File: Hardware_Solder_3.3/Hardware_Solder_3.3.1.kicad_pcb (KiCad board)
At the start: 2 copper layers, 86.5 x 47.4 mm, 95 parts, among them J1 Connector, J2 POWER, J3 SENSOR, J4 BATTERY, J5 Control Panel, J6 SWD DEBUG, J7 HEAT_WIRE, Q1 S8050, Q2 S8050, Q3 S8550, Q4 IRFS4227, Q6 S8050, SW1 RESET, U1 LM358, U2 W25Q32JVSS, U3 LM2596S-ADJ, U4 ACS712-05A, U5 AMS1117-3.3, U6 STM32F103C8Tx, Y1 32.768KHz, Y2 8MHz

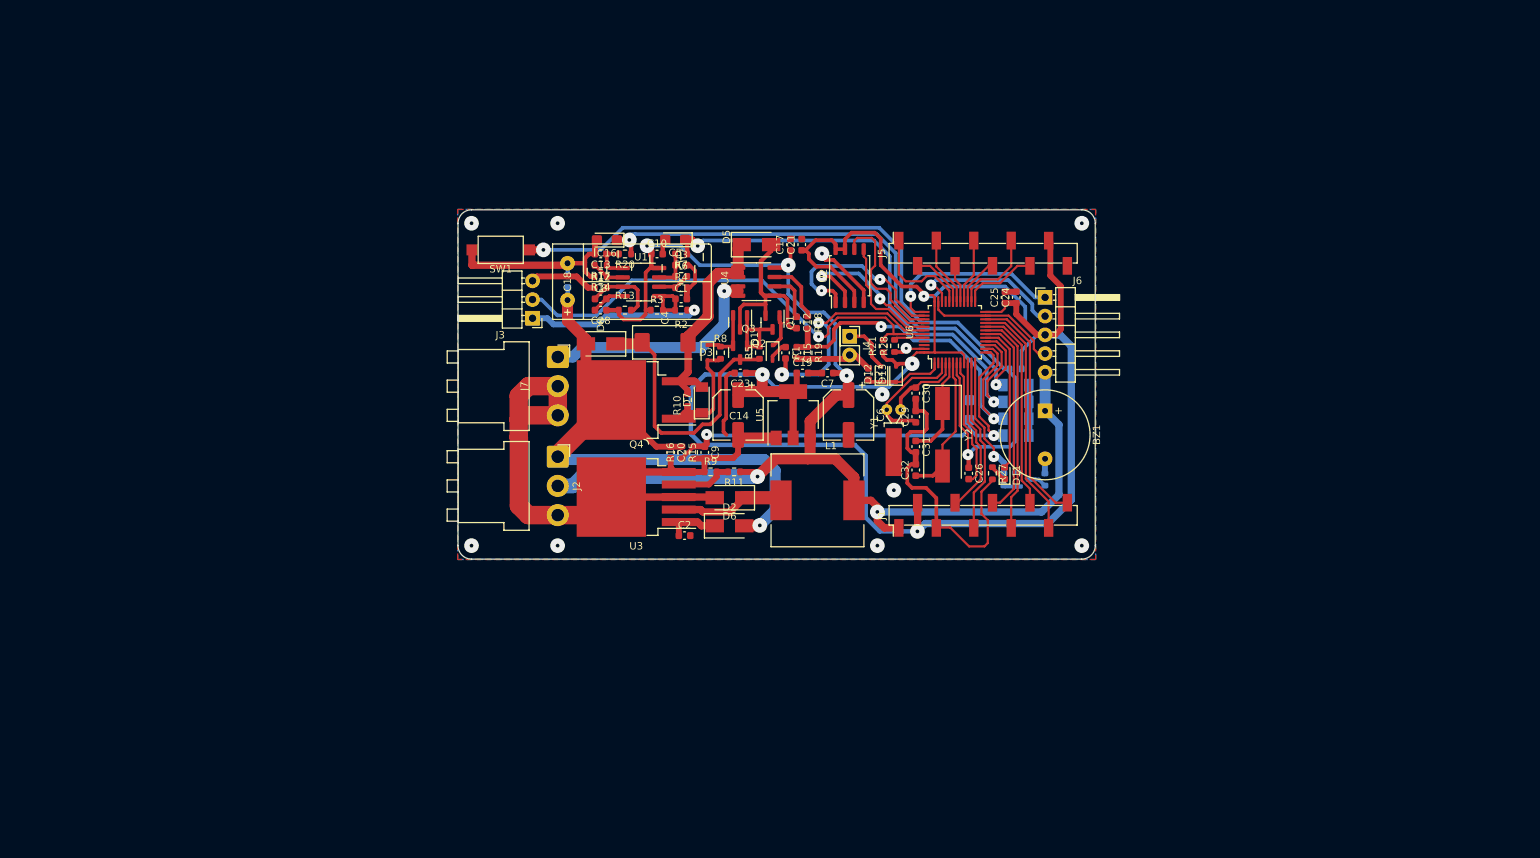
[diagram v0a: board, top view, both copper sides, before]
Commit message: Add files via upload
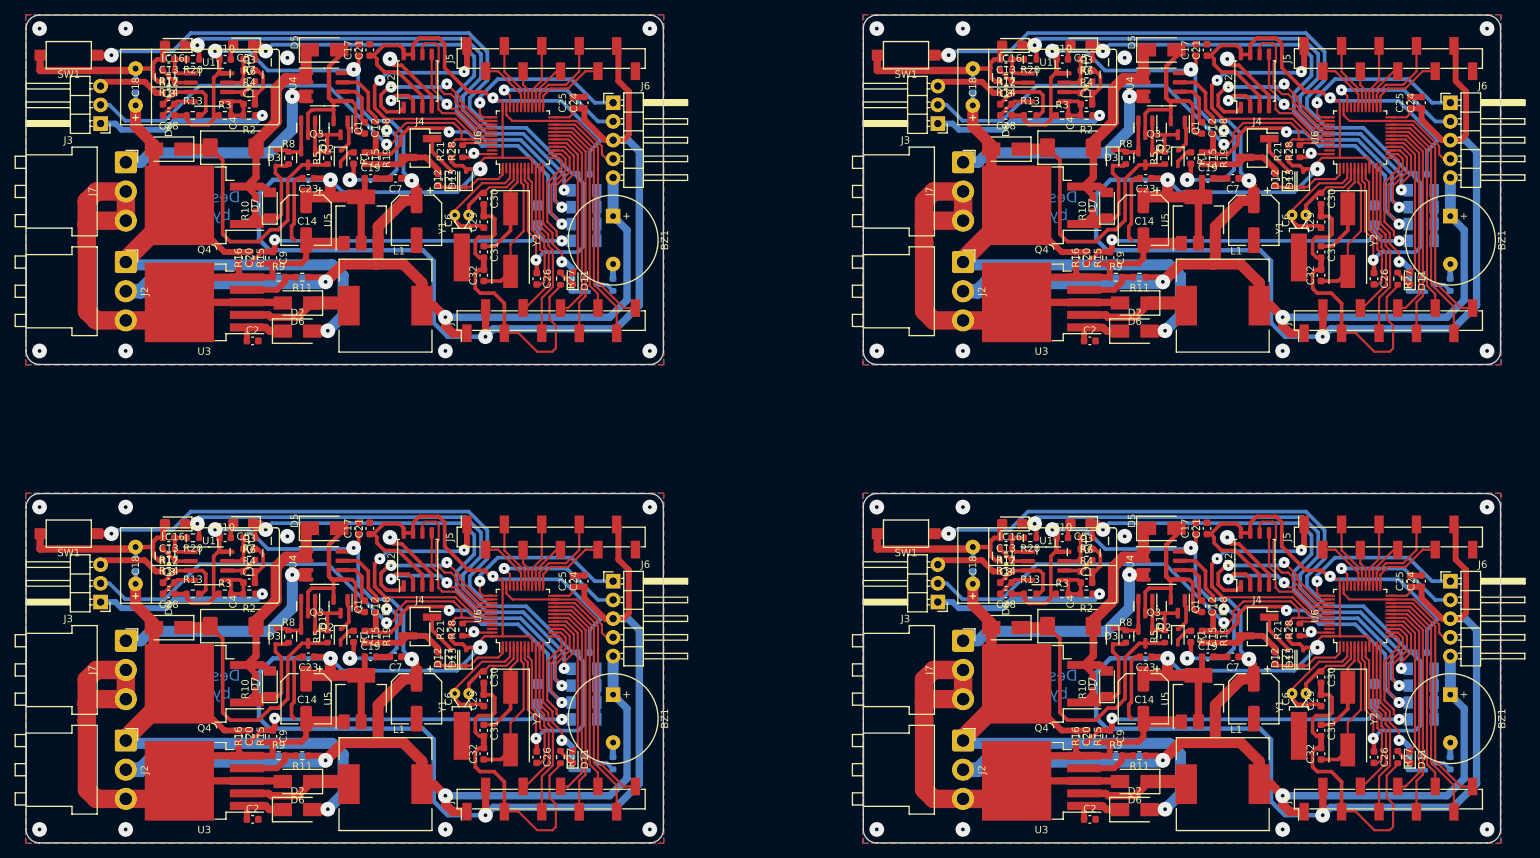
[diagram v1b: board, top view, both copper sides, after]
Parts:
- added BZ1: Buzzer, Buzzer_Beeper:MagneticBuzzer_ProSignal_ABT-410-RC, F.Cu at (127.7, 66.9)
- added BZ1: Buzzer, Buzzer_Beeper:MagneticBuzzer_ProSignal_ABT-410-RC, F.Cu at (127.7, 131.8)
- added BZ1: Buzzer, Buzzer_Beeper:MagneticBuzzer_ProSignal_ABT-410-RC, F.Cu at (241.3, 66.9)
- added C1: 0.1uF, Capacitor_SMD:C_0603_1608Metric, F.Cu at (78.3, 116.6)
- added C1: 0.1uF, Capacitor_SMD:C_0603_1608Metric, F.Cu at (191.9, 51.7)
- added C1: 0.1uF, Capacitor_SMD:C_0603_1608Metric, F.Cu at (78.3, 51.7)
- added C10: 0.1uF, Capacitor_SMD:C_0603_1608Metric, F.Cu at (188.7, 45.6)
- added C10: 0.1uF, Capacitor_SMD:C_0603_1608Metric, F.Cu at (75.1, 110.5)
- added C10: 0.1uF, Capacitor_SMD:C_0603_1608Metric, F.Cu at (75.1, 45.6)
- added C11: 4.7uF, Capacitor_Tantalum_SMD:CP_EIA-3216-12_Kemet-S, B.Cu at (231.1, 66.8)
- added C11: 4.7uF, Capacitor_Tantalum_SMD:CP_EIA-3216-12_Kemet-S, B.Cu at (117.5, 66.8)
- added C11: 4.7uF, Capacitor_Tantalum_SMD:CP_EIA-3216-12_Kemet-S, B.Cu at (117.5, 131.7)
- added C12: 0.1nF, Capacitor_SMD:C_0603_1608Metric, F.Cu at (94.0, 119.8)
- added C12: 0.1nF, Capacitor_SMD:C_0603_1608Metric, F.Cu at (94.0, 54.9)
- added C12: 0.1nF, Capacitor_SMD:C_0603_1608Metric, F.Cu at (207.6, 54.9)
- added C13: 0.1uF, Capacitor_SMD:C_0603_1608Metric, F.Cu at (67.4, 110.5)
- added C13: 0.1uF, Capacitor_SMD:C_0603_1608Metric, F.Cu at (67.4, 45.6)
- added C13: 0.1uF, Capacitor_SMD:C_0603_1608Metric, F.Cu at (181.0, 45.6)
- added C14: 220uF, Capacitor_SMD:CP_Elec_6.3x7.7, F.Cu at (86.1, 67.5)
- added C14: 220uF, Capacitor_SMD:CP_Elec_6.3x7.7, F.Cu at (199.7, 67.5)
- added C14: 220uF, Capacitor_SMD:CP_Elec_6.3x7.7, F.Cu at (86.1, 132.4)
- added C15: 0.1uF, Capacitor_SMD:C_0603_1608Metric, F.Cu at (207.6, 59.0)
- added C15: 0.1uF, Capacitor_SMD:C_0603_1608Metric, F.Cu at (94.0, 59.0)
- added C15: 0.1uF, Capacitor_SMD:C_0603_1608Metric, F.Cu at (94.0, 124.0)
- added C16: 4.7uF, Capacitor_Tantalum_SMD:CP_EIA-3216-12_Kemet-S, F.Cu at (68.3, 108.7)
- added C16: 4.7uF, Capacitor_Tantalum_SMD:CP_EIA-3216-12_Kemet-S, F.Cu at (68.3, 43.7)
- added C16: 4.7uF, Capacitor_Tantalum_SMD:CP_EIA-3216-12_Kemet-S, F.Cu at (181.9, 43.7)
- added C17: 0.1uF, Capacitor_SMD:C_0603_1608Metric, F.Cu at (206.8, 44.3)
- added C17: 0.1uF, Capacitor_SMD:C_0603_1608Metric, F.Cu at (93.2, 44.3)
- added C17: 0.1uF, Capacitor_SMD:C_0603_1608Metric, F.Cu at (93.2, 109.3)
- added C18: 470uF, Capacitor_THT:C_Radial_D10.0mm_H20.0mm_P5.00mm, F.Cu at (176.5, 51.9)
- added C18: 470uF, Capacitor_THT:C_Radial_D10.0mm_H20.0mm_P5.00mm, F.Cu at (62.9, 116.8)
- added C18: 470uF, Capacitor_THT:C_Radial_D10.0mm_H20.0mm_P5.00mm, F.Cu at (62.9, 51.9)
- added C19: 0.1uF, Capacitor_SMD:C_0603_1608Metric, F.Cu at (208.4, 61.8)
- added C19: 0.1uF, Capacitor_SMD:C_0603_1608Metric, F.Cu at (94.8, 61.8)
- added C19: 0.1uF, Capacitor_SMD:C_0603_1608Metric, F.Cu at (94.8, 126.7)
- added C2: 0.1uF, Capacitor_SMD:C_0603_1608Metric, F.Cu at (192.4, 83.8)
- added C2: 0.1uF, Capacitor_SMD:C_0603_1608Metric, F.Cu at (78.8, 83.8)
- added C2: 0.1uF, Capacitor_SMD:C_0603_1608Metric, F.Cu at (78.8, 148.8)
- added C20: 0.1uF, Capacitor_SMD:C_0603_1608Metric, F.Cu at (76.9, 72.5)
- added C20: 0.1uF, Capacitor_SMD:C_0603_1608Metric, F.Cu at (76.9, 137.5)
- added C20: 0.1uF, Capacitor_SMD:C_0603_1608Metric, F.Cu at (190.5, 72.5)
- added C21: 0.1uF, Capacitor_SMD:C_0603_1608Metric, F.Cu at (94.7, 44.3)
- added C21: 0.1uF, Capacitor_SMD:C_0603_1608Metric, F.Cu at (208.3, 44.3)
- added C21: 0.1uF, Capacitor_SMD:C_0603_1608Metric, F.Cu at (94.7, 109.3)
- added C22: 0.1uF, Capacitor_SMD:C_0603_1608Metric, B.Cu at (63.0, 49.4)
- added C22: 0.1uF, Capacitor_SMD:C_0603_1608Metric, B.Cu at (176.6, 49.4)
- added C22: 0.1uF, Capacitor_SMD:C_0603_1608Metric, B.Cu at (63.0, 114.3)
- added C23: 0.1uF, Capacitor_SMD:C_0603_1608Metric, F.Cu at (86.4, 61.8)
- added C23: 0.1uF, Capacitor_SMD:C_0603_1608Metric, F.Cu at (86.4, 126.7)
- added C23: 0.1uF, Capacitor_SMD:C_0603_1608Metric, F.Cu at (200.0, 61.8)
- added C24: 0.1uF, Capacitor_SMD:C_0603_1608Metric, F.Cu at (123.8, 51.5)
- added C24: 0.1uF, Capacitor_SMD:C_0603_1608Metric, F.Cu at (237.4, 51.5)
- added C24: 0.1uF, Capacitor_SMD:C_0603_1608Metric, F.Cu at (123.8, 116.4)
- added C25: 0.1uF, Capacitor_SMD:C_0603_1608Metric, F.Cu at (235.9, 51.5)
- added C25: 0.1uF, Capacitor_SMD:C_0603_1608Metric, F.Cu at (122.3, 51.5)
- added C25: 0.1uF, Capacitor_SMD:C_0603_1608Metric, F.Cu at (122.3, 116.4)
- added C26: 0.1uF, Capacitor_SMD:C_0603_1608Metric, F.Cu at (117.4, 75.4)
- added C26: 0.1uF, Capacitor_SMD:C_0603_1608Metric, F.Cu at (231.0, 75.4)
- added C26: 0.1uF, Capacitor_SMD:C_0603_1608Metric, F.Cu at (117.4, 140.3)
- added C27: 0.1uF, Capacitor_SMD:C_0603_1608Metric, F.Cu at (104.0, 126.8)
- added C27: 0.1uF, Capacitor_SMD:C_0603_1608Metric, F.Cu at (217.6, 61.9)
- added C27: 0.1uF, Capacitor_SMD:C_0603_1608Metric, F.Cu at (104.0, 61.9)
- added C28: 0.1uF, Capacitor_SMD:C_0603_1608Metric, F.Cu at (67.4, 53.2)
- added C28: 0.1uF, Capacitor_SMD:C_0603_1608Metric, F.Cu at (67.4, 118.2)
- added C28: 0.1uF, Capacitor_SMD:C_0603_1608Metric, F.Cu at (181.0, 53.2)
- added C29: 22pF, Capacitor_SMD:C_0603_1608Metric, F.Cu at (110.2, 132.6)
- added C29: 22pF, Capacitor_SMD:C_0603_1608Metric, F.Cu at (223.8, 67.7)
- added C29: 22pF, Capacitor_SMD:C_0603_1608Metric, F.Cu at (110.2, 67.7)
- added C3: 0.1uF, Capacitor_SMD:C_0603_1608Metric, F.Cu at (78.3, 47.1)
- added C3: 0.1uF, Capacitor_SMD:C_0603_1608Metric, F.Cu at (78.3, 112.1)
- added C3: 0.1uF, Capacitor_SMD:C_0603_1608Metric, F.Cu at (191.9, 47.1)
- added C30: 22pF, Capacitor_SMD:C_0603_1608Metric, F.Cu at (110.2, 129.4)
- added C30: 22pF, Capacitor_SMD:C_0603_1608Metric, F.Cu at (223.8, 64.5)
- added C30: 22pF, Capacitor_SMD:C_0603_1608Metric, F.Cu at (110.2, 64.5)
- added C31: 22pF, Capacitor_SMD:C_0603_1608Metric, F.Cu at (110.2, 71.8)
- added C31: 22pF, Capacitor_SMD:C_0603_1608Metric, F.Cu at (110.2, 136.7)
- added C31: 22pF, Capacitor_SMD:C_0603_1608Metric, F.Cu at (223.8, 71.8)
- added C32: 22pF, Capacitor_SMD:C_0603_1608Metric, F.Cu at (223.8, 74.9)
- added C32: 22pF, Capacitor_SMD:C_0603_1608Metric, F.Cu at (110.2, 74.9)
- added C32: 22pF, Capacitor_SMD:C_0603_1608Metric, F.Cu at (110.2, 139.9)
- added C4: 22uF, Capacitor_Tantalum_SMD:CP_EIA-7343-43_Kemet-X, F.Cu at (76.2, 122.5)
- added C4: 22uF, Capacitor_Tantalum_SMD:CP_EIA-7343-43_Kemet-X, F.Cu at (76.2, 57.6)
- added C4: 22uF, Capacitor_Tantalum_SMD:CP_EIA-7343-43_Kemet-X, F.Cu at (189.8, 57.6)
- added C5: 4.7uF, Capacitor_Tantalum_SMD:CP_EIA-3216-12_Kemet-S, F.Cu at (191.1, 43.7)
- added C5: 4.7uF, Capacitor_Tantalum_SMD:CP_EIA-3216-12_Kemet-S, F.Cu at (77.5, 43.7)
- added C5: 4.7uF, Capacitor_Tantalum_SMD:CP_EIA-3216-12_Kemet-S, F.Cu at (77.5, 108.6)
- added C6: 220uF, Capacitor_SMD:CP_Elec_6.3x7.7, F.Cu at (101.1, 67.5)
- added C6: 220uF, Capacitor_SMD:CP_Elec_6.3x7.7, F.Cu at (214.7, 67.5)
- added C6: 220uF, Capacitor_SMD:CP_Elec_6.3x7.7, F.Cu at (101.1, 132.4)
- added C7: 0.1uF, Capacitor_SMD:C_0603_1608Metric, F.Cu at (211.8, 61.8)
- added C7: 0.1uF, Capacitor_SMD:C_0603_1608Metric, F.Cu at (98.2, 61.8)
- added C7: 0.1uF, Capacitor_SMD:C_0603_1608Metric, F.Cu at (98.2, 126.7)
- added C8: 0.1uF, Capacitor_SMD:C_0603_1608Metric, F.Cu at (67.4, 116.6)
- added C8: 0.1uF, Capacitor_SMD:C_0603_1608Metric, F.Cu at (67.4, 51.7)
- added C8: 0.1uF, Capacitor_SMD:C_0603_1608Metric, F.Cu at (181.0, 51.7)
- added C9: 0.1uF, Capacitor_SMD:C_0603_1608Metric, F.Cu at (81.5, 72.5)
- added C9: 0.1uF, Capacitor_SMD:C_0603_1608Metric, F.Cu at (195.1, 72.5)
- added C9: 0.1uF, Capacitor_SMD:C_0603_1608Metric, F.Cu at (81.5, 137.5)
- added D1: 1N4148WS, Diode_SMD:D_SOD-323, F.Cu at (90.7, 124.0)
- added D1: 1N4148WS, Diode_SMD:D_SOD-323, F.Cu at (204.3, 59.0)
- added D1: 1N4148WS, Diode_SMD:D_SOD-323, F.Cu at (90.7, 59.0)
- added D10: Z3.3V, Diode_SMD:D_MiniMELF, B.Cu at (123.8, 132.9)
- added D10: Z3.3V, Diode_SMD:D_MiniMELF, B.Cu at (123.8, 68.0)
- added D10: Z3.3V, Diode_SMD:D_MiniMELF, B.Cu at (237.4, 68.0)
- added D11: LED, LED_SMD:LED_0603_1608Metric, F.Cu at (235.8, 75.4)
- added D11: LED, LED_SMD:LED_0603_1608Metric, F.Cu at (122.2, 75.4)
- added D11: LED, LED_SMD:LED_0603_1608Metric, F.Cu at (122.2, 140.3)
- added D12: 1N4148WS, Diode_SMD:D_SOD-323, F.Cu at (105.8, 61.9)
- added D12: 1N4148WS, Diode_SMD:D_SOD-323, F.Cu at (105.8, 126.8)
- added D12: 1N4148WS, Diode_SMD:D_SOD-323, F.Cu at (219.4, 61.9)
- added D13: 1N4148WS, Diode_SMD:D_SOD-323, F.Cu at (107.8, 126.8)
- added D13: 1N4148WS, Diode_SMD:D_SOD-323, F.Cu at (221.4, 61.9)
- added D13: 1N4148WS, Diode_SMD:D_SOD-323, F.Cu at (107.8, 61.9)
- added D14: Z3.3V, Diode_SMD:D_MiniMELF, B.Cu at (123.8, 135.2)
- added D14: Z3.3V, Diode_SMD:D_MiniMELF, B.Cu at (123.8, 70.3)
- added D14: Z3.3V, Diode_SMD:D_MiniMELF, B.Cu at (237.4, 70.3)
- added D2: SS34, Diode_SMD:D_SMA, F.Cu at (84.9, 147.4)
- added D2: SS34, Diode_SMD:D_SMA, F.Cu at (198.5, 82.5)
- added D2: SS34, Diode_SMD:D_SMA, F.Cu at (84.9, 82.5)
- added D3: 1N4148WS, Diode_SMD:D_SOD-323, F.Cu at (195.5, 59.0)
- added D3: 1N4148WS, Diode_SMD:D_SOD-323, F.Cu at (81.9, 123.9)
- added D3: 1N4148WS, Diode_SMD:D_SOD-323, F.Cu at (81.9, 59.0)
- added D4: Z3.3V, Diode_SMD:D_MiniMELF, B.Cu at (237.4, 65.7)
- added D4: Z3.3V, Diode_SMD:D_MiniMELF, B.Cu at (123.8, 130.6)
- added D4: Z3.3V, Diode_SMD:D_MiniMELF, B.Cu at (123.8, 65.7)
- added D5: SS34, Diode_SMD:D_SMA, F.Cu at (88.6, 109.3)
- added D5: SS34, Diode_SMD:D_SMA, F.Cu at (88.6, 44.3)
- added D5: SS34, Diode_SMD:D_SMA, F.Cu at (202.2, 44.3)
- added D6: SS34, Diode_SMD:D_SMA, F.Cu at (198.5, 78.7)
- added D6: SS34, Diode_SMD:D_SMA, F.Cu at (84.9, 143.6)
- added D6: SS34, Diode_SMD:D_SMA, F.Cu at (84.9, 78.7)
- added D7: Z18V, Diode_SMD:D_MiniMELF, F.Cu at (81.1, 130.4)
- added D7: Z18V, Diode_SMD:D_MiniMELF, F.Cu at (81.1, 65.4)
- added D7: Z18V, Diode_SMD:D_MiniMELF, F.Cu at (194.7, 65.4)
- added D8: SS14, Diode_SMD:D_SMA, F.Cu at (181.0, 57.8)
- added D8: SS14, Diode_SMD:D_SMA, F.Cu at (67.4, 122.7)
- added D8: SS14, Diode_SMD:D_SMA, F.Cu at (67.4, 57.8)
- added D9: Z3.3V, Diode_SMD:D_MiniMELF, B.Cu at (123.8, 128.3)
- added D9: Z3.3V, Diode_SMD:D_MiniMELF, B.Cu at (123.8, 63.4)
- added D9: Z3.3V, Diode_SMD:D_MiniMELF, B.Cu at (237.4, 63.4)
- added J1: Connector, Connector_PinHeader_2.54mm:PinHeader_1x10_P2.54mm_Vertical_SMD_Pin1Left, F.Cu at (119.3, 146.0)
- added J1: Connector, Connector_PinHeader_2.54mm:PinHeader_1x10_P2.54mm_Vertical_SMD_Pin1Left, F.Cu at (232.9, 81.1)
- added J1: Connector, Connector_PinHeader_2.54mm:PinHeader_1x10_P2.54mm_Vertical_SMD_Pin1Left, F.Cu at (119.3, 81.1)
- added J2: POWER, Connector_JST:JST_VH_B3PS-VH_1x03_P3.96mm_Horizontal, F.Cu at (175.2, 73.1)
- added J2: POWER, Connector_JST:JST_VH_B3PS-VH_1x03_P3.96mm_Horizontal, F.Cu at (61.6, 73.1)
- added J2: POWER, Connector_JST:JST_VH_B3PS-VH_1x03_P3.96mm_Horizontal, F.Cu at (61.6, 138.1)
- added J3: SENSOR, Connector_PinHeader_2.54mm:PinHeader_1x03_P2.54mm_Horizontal, F.Cu at (58.2, 54.3)
- added J3: SENSOR, Connector_PinHeader_2.54mm:PinHeader_1x03_P2.54mm_Horizontal, F.Cu at (58.2, 119.3)
- added J3: SENSOR, Connector_PinHeader_2.54mm:PinHeader_1x03_P2.54mm_Horizontal, F.Cu at (171.8, 54.3)
- added J4: BATTERY, Connector_PinHeader_2.54mm:PinHeader_1x02_P2.54mm_Vertical_SMD_Pin1Right, F.Cu at (101.5, 57.7)
- added J4: BATTERY, Connector_PinHeader_2.54mm:PinHeader_1x02_P2.54mm_Vertical_SMD_Pin1Right, F.Cu at (215.1, 57.7)
- added J4: BATTERY, Connector_PinHeader_2.54mm:PinHeader_1x02_P2.54mm_Vertical_SMD_Pin1Right, F.Cu at (101.5, 122.6)
- added J5: Control Panel, Connector_PinHeader_2.54mm:PinHeader_1x10_P2.54mm_Vertical_SMD_Pin1Right, F.Cu at (119.3, 45.5)
- added J5: Control Panel, Connector_PinHeader_2.54mm:PinHeader_1x10_P2.54mm_Vertical_SMD_Pin1Right, F.Cu at (232.9, 45.5)
- added J5: Control Panel, Connector_PinHeader_2.54mm:PinHeader_1x10_P2.54mm_Vertical_SMD_Pin1Right, F.Cu at (119.3, 110.4)
- added J6: SWD DEBUG, Connector_PinHeader_2.54mm:PinHeader_1x05_P2.54mm_Horizontal, F.Cu at (127.7, 51.5)
- added J6: SWD DEBUG, Connector_PinHeader_2.54mm:PinHeader_1x05_P2.54mm_Horizontal, F.Cu at (241.3, 51.5)
- added J6: SWD DEBUG, Connector_PinHeader_2.54mm:PinHeader_1x05_P2.54mm_Horizontal, F.Cu at (127.7, 116.4)
- added J7: HEAT_WIRE, Connector_JST:JST_VH_B3PS-VH_1x03_P3.96mm_Horizontal, F.Cu at (61.6, 59.6)
- added J7: HEAT_WIRE, Connector_JST:JST_VH_B3PS-VH_1x03_P3.96mm_Horizontal, F.Cu at (175.2, 59.6)
- added J7: HEAT_WIRE, Connector_JST:JST_VH_B3PS-VH_1x03_P3.96mm_Horizontal, F.Cu at (61.6, 124.5)
- added L1: 47uH, Inductor_SMD:L_12x12mm_H8mm, F.Cu at (210.4, 79.0)
- added L1: 47uH, Inductor_SMD:L_12x12mm_H8mm, F.Cu at (96.8, 144.0)
- added L1: 47uH, Inductor_SMD:L_12x12mm_H8mm, F.Cu at (96.8, 79.0)
- added Q1: S8050, Package_TO_SOT_SMD:SOT-23, F.Cu at (90.7, 54.9)
- added Q1: S8050, Package_TO_SOT_SMD:SOT-23, F.Cu at (90.7, 119.8)
- added Q1: S8050, Package_TO_SOT_SMD:SOT-23, F.Cu at (204.3, 54.9)
- added Q2: S8050, Package_TO_SOT_SMD:SOT-23, F.Cu at (86.3, 123.9)
- added Q2: S8050, Package_TO_SOT_SMD:SOT-23, F.Cu at (86.3, 59.0)
- added Q2: S8050, Package_TO_SOT_SMD:SOT-23, F.Cu at (199.9, 59.0)
- added Q3: S8550, Package_TO_SOT_SMD:SOT-23, F.Cu at (86.3, 54.9)
- added Q3: S8550, Package_TO_SOT_SMD:SOT-23, F.Cu at (199.9, 54.9)
- added Q3: S8550, Package_TO_SOT_SMD:SOT-23, F.Cu at (86.3, 119.8)
- added Q4: IRFS4227, Package_TO_SOT_SMD:TO-263-2, F.Cu at (72.2, 65.4)
- added Q4: IRFS4227, Package_TO_SOT_SMD:TO-263-2, F.Cu at (185.8, 65.4)
- added Q4: IRFS4227, Package_TO_SOT_SMD:TO-263-2, F.Cu at (72.2, 130.4)
- added Q6: S8050, Package_TO_SOT_SMD:SOT-23, B.Cu at (124.9, 141.1)
- added Q6: S8050, Package_TO_SOT_SMD:SOT-23, B.Cu at (124.9, 76.2)
- added Q6: S8050, Package_TO_SOT_SMD:SOT-23, B.Cu at (238.5, 76.2)
- added R1: 5k6, Capacitor_SMD:C_0603_1608Metric, F.Cu at (92.5, 124.0)
- added R1: 5k6, Capacitor_SMD:C_0603_1608Metric, F.Cu at (206.1, 59.0)
- added R1: 5k6, Capacitor_SMD:C_0603_1608Metric, F.Cu at (92.5, 59.0)
- added R10: 5k6, Resistor_SMD:R_0603_1608Metric, F.Cu at (79.2, 130.4)
- added R10: 5k6, Resistor_SMD:R_0603_1608Metric, F.Cu at (192.8, 65.4)
- added R10: 5k6, Resistor_SMD:R_0603_1608Metric, F.Cu at (79.2, 65.4)
- added R11: 3k, Resistor_SMD:R_0603_1608Metric, F.Cu at (85.5, 75.2)
- added R11: 3k, Resistor_SMD:R_0603_1608Metric, F.Cu at (85.5, 140.1)
- added R11: 3k, Resistor_SMD:R_0603_1608Metric, F.Cu at (199.1, 75.2)
- added R12: 50, Resistor_SMD:R_0603_1608Metric, F.Cu at (181.0, 50.2)
- added R12: 50, Resistor_SMD:R_0603_1608Metric, F.Cu at (67.4, 115.1)
- added R12: 50, Resistor_SMD:R_0603_1608Metric, F.Cu at (67.4, 50.2)
- added R13: 1k, Resistor_SMD:R_0603_1608Metric, F.Cu at (70.7, 53.2)
- added R13: 1k, Resistor_SMD:R_0603_1608Metric, F.Cu at (70.7, 118.2)
- added R13: 1k, Resistor_SMD:R_0603_1608Metric, F.Cu at (184.3, 53.2)
- added R14: 1k, Resistor_SMD:R_0603_1608Metric, F.Cu at (181.0, 48.7)
- added R14: 1k, Resistor_SMD:R_0603_1608Metric, F.Cu at (67.4, 113.6)
- added R14: 1k, Resistor_SMD:R_0603_1608Metric, F.Cu at (67.4, 48.7)
- added R15: 15k, Resistor_SMD:R_0603_1608Metric, F.Cu at (192.0, 72.5)
- added R15: 15k, Resistor_SMD:R_0603_1608Metric, F.Cu at (78.4, 137.5)
- added R15: 15k, Resistor_SMD:R_0603_1608Metric, F.Cu at (78.4, 72.5)
- added R16: 1k, Resistor_SMD:R_0603_1608Metric, F.Cu at (80.0, 72.5)
- added R16: 1k, Resistor_SMD:R_0603_1608Metric, F.Cu at (193.6, 72.5)
- added R16: 1k, Resistor_SMD:R_0603_1608Metric, F.Cu at (80.0, 137.5)
- added R17: 1.5k, Resistor_SMD:R_0603_1608Metric, F.Cu at (67.4, 112.1)
- added R17: 1.5k, Resistor_SMD:R_0603_1608Metric, F.Cu at (181.0, 47.1)
- added R17: 1.5k, Resistor_SMD:R_0603_1608Metric, F.Cu at (67.4, 47.1)
- added R18: 470, Resistor_SMD:R_0603_1608Metric, F.Cu at (95.5, 119.8)
- added R18: 470, Resistor_SMD:R_0603_1608Metric, F.Cu at (209.1, 54.9)
- added R18: 470, Resistor_SMD:R_0603_1608Metric, F.Cu at (95.5, 54.9)
- added R19: 1k, Resistor_SMD:R_0603_1608Metric, F.Cu at (95.6, 124.0)
- added R19: 1k, Resistor_SMD:R_0603_1608Metric, F.Cu at (95.6, 59.0)
- added R19: 1k, Resistor_SMD:R_0603_1608Metric, F.Cu at (209.2, 59.0)
- added R2: 5k, Resistor_SMD:R_0603_1608Metric, F.Cu at (191.9, 53.2)
- added R2: 5k, Resistor_SMD:R_0603_1608Metric, F.Cu at (78.3, 118.2)
- added R2: 5k, Resistor_SMD:R_0603_1608Metric, F.Cu at (78.3, 53.2)
- added R20: 220, Resistor_SMD:R_0603_1608Metric, F.Cu at (70.7, 45.6)
- added R20: 220, Resistor_SMD:R_0603_1608Metric, F.Cu at (70.7, 110.5)
- added R20: 220, Resistor_SMD:R_0603_1608Metric, F.Cu at (184.3, 45.6)
- added R21: 10k, Resistor_SMD:R_0603_1608Metric, F.Cu at (219.4, 58.1)
- added R21: 10k, Resistor_SMD:R_0603_1608Metric, F.Cu at (105.8, 123.0)
- added R21: 10k, Resistor_SMD:R_0603_1608Metric, F.Cu at (105.8, 58.1)
- added R24: 1k, Resistor_SMD:R_0603_1608Metric, B.Cu at (122.1, 141.1)
- added R24: 1k, Resistor_SMD:R_0603_1608Metric, B.Cu at (235.7, 76.2)
- added R24: 1k, Resistor_SMD:R_0603_1608Metric, B.Cu at (122.1, 76.2)
- added R25: 220, Resistor_SMD:R_0603_1608Metric, B.Cu at (127.7, 141.1)
- added R25: 220, Resistor_SMD:R_0603_1608Metric, B.Cu at (241.3, 76.2)
- added R25: 220, Resistor_SMD:R_0603_1608Metric, B.Cu at (127.7, 76.2)
- added R26: 10k, Resistor_SMD:R_0603_1608Metric, B.Cu at (123.7, 126.1)
- added R26: 10k, Resistor_SMD:R_0603_1608Metric, B.Cu at (123.7, 61.2)
- added R26: 10k, Resistor_SMD:R_0603_1608Metric, B.Cu at (237.3, 61.2)
- added R27: 220, Resistor_SMD:R_0603_1608Metric, F.Cu at (120.6, 140.3)
- added R27: 220, Resistor_SMD:R_0603_1608Metric, F.Cu at (120.6, 75.4)
- added R27: 220, Resistor_SMD:R_0603_1608Metric, F.Cu at (234.2, 75.4)
- added R28: 1k, Resistor_SMD:R_0603_1608Metric, F.Cu at (107.3, 123.0)
- added R28: 1k, Resistor_SMD:R_0603_1608Metric, F.Cu at (220.9, 58.1)
- added R28: 1k, Resistor_SMD:R_0603_1608Metric, F.Cu at (107.3, 58.1)
- added R3: 10k, Resistor_SMD:R_0603_1608Metric, F.Cu at (75.0, 53.2)
- added R3: 10k, Resistor_SMD:R_0603_1608Metric, F.Cu at (188.6, 53.2)
- added R3: 10k, Resistor_SMD:R_0603_1608Metric, F.Cu at (75.0, 118.2)
- added R4: 1k, Resistor_SMD:R_0603_1608Metric, F.Cu at (78.3, 115.1)
- added R4: 1k, Resistor_SMD:R_0603_1608Metric, F.Cu at (78.3, 50.2)
- added R4: 1k, Resistor_SMD:R_0603_1608Metric, F.Cu at (191.9, 50.2)
- added R5: 5k6, Resistor_SMD:R_0603_1608Metric, F.Cu at (202.6, 59.0)
- added R5: 5k6, Resistor_SMD:R_0603_1608Metric, F.Cu at (89.0, 123.9)
- added R5: 5k6, Resistor_SMD:R_0603_1608Metric, F.Cu at (89.0, 59.0)
- added R6: 1k, Resistor_SMD:R_0603_1608Metric, F.Cu at (78.3, 113.6)
- added R6: 1k, Resistor_SMD:R_0603_1608Metric, F.Cu at (191.9, 48.7)
- added R6: 1k, Resistor_SMD:R_0603_1608Metric, F.Cu at (78.3, 48.7)
- added R7: 220, Resistor_SMD:R_0603_1608Metric, F.Cu at (191.9, 45.6)
- added R7: 220, Resistor_SMD:R_0603_1608Metric, F.Cu at (78.3, 110.5)
- added R7: 220, Resistor_SMD:R_0603_1608Metric, F.Cu at (78.3, 45.6)
- added R8: 10, Resistor_SMD:R_0603_1608Metric, F.Cu at (197.3, 59.0)
- added R8: 10, Resistor_SMD:R_0603_1608Metric, F.Cu at (83.7, 123.9)
- added R8: 10, Resistor_SMD:R_0603_1608Metric, F.Cu at (83.7, 59.0)
- added R9: 1k, Resistor_SMD:R_0603_1608Metric, F.Cu at (195.9, 75.2)
- added R9: 1k, Resistor_SMD:R_0603_1608Metric, F.Cu at (82.3, 75.2)
- added R9: 1k, Resistor_SMD:R_0603_1608Metric, F.Cu at (82.3, 140.1)
- added SW1: RESET, Button_Switch_SMD:SW_SPST_CK_RS282G05A3, F.Cu at (167.5, 45.1)
- added SW1: RESET, Button_Switch_SMD:SW_SPST_CK_RS282G05A3, F.Cu at (53.9, 45.1)
- added SW1: RESET, Button_Switch_SMD:SW_SPST_CK_RS282G05A3, F.Cu at (53.9, 110.0)
- added U1: LM358, Package_SO:SOIC-8_3.9x4.9mm_P1.27mm, F.Cu at (72.9, 49.4)
- added U1: LM358, Package_SO:SOIC-8_3.9x4.9mm_P1.27mm, F.Cu at (186.5, 49.4)
- added U1: LM358, Package_SO:SOIC-8_3.9x4.9mm_P1.27mm, F.Cu at (72.9, 114.4)
- added U2: W25Q32JVSS, Package_SO:SOIC-8_5.23x5.23mm_P1.27mm, F.Cu at (214.8, 48.6)
- added U2: W25Q32JVSS, Package_SO:SOIC-8_5.23x5.23mm_P1.27mm, F.Cu at (101.2, 48.6)
- added U2: W25Q32JVSS, Package_SO:SOIC-8_5.23x5.23mm_P1.27mm, F.Cu at (101.2, 113.5)
- added U3: LM2596S-ADJ, Package_TO_SOT_SMD:TO-263-5_TabPin3, F.Cu at (72.2, 78.6)
- added U3: LM2596S-ADJ, Package_TO_SOT_SMD:TO-263-5_TabPin3, F.Cu at (185.8, 78.6)
- added U3: LM2596S-ADJ, Package_TO_SOT_SMD:TO-263-5_TabPin3, F.Cu at (72.2, 143.5)
- added U4: ACS712-05A, Package_SO:SOIC-8_3.9x4.9mm_P1.27mm, F.Cu at (88.6, 49.4)
- added U4: ACS712-05A, Package_SO:SOIC-8_3.9x4.9mm_P1.27mm, F.Cu at (202.2, 49.4)
- added U4: ACS712-05A, Package_SO:SOIC-8_3.9x4.9mm_P1.27mm, F.Cu at (88.6, 114.3)
- added U5: AMS1117-3.3, Package_TO_SOT_SMD:SOT-223-3_TabPin2, F.Cu at (207.1, 67.4)
- added U5: AMS1117-3.3, Package_TO_SOT_SMD:SOT-223-3_TabPin2, F.Cu at (93.5, 67.4)
- added U5: AMS1117-3.3, Package_TO_SOT_SMD:SOT-223-3_TabPin2, F.Cu at (93.5, 132.4)
- added U6: STM32F103C8Tx, Package_QFP:LQFP-48_7x7mm_P0.5mm, F.Cu at (229.1, 56.2)
- added U6: STM32F103C8Tx, Package_QFP:LQFP-48_7x7mm_P0.5mm, F.Cu at (115.5, 121.2)
- added U6: STM32F103C8Tx, Package_QFP:LQFP-48_7x7mm_P0.5mm, F.Cu at (115.5, 56.2)
- added Y1: 32.768KHz, Crystal:Crystal_C26-LF_D2.1mm_L6.5mm_Horizontal_1EP_style1, F.Cu at (106.2, 131.7)
- added Y1: 32.768KHz, Crystal:Crystal_C26-LF_D2.1mm_L6.5mm_Horizontal_1EP_style1, F.Cu at (106.2, 66.8)
- added Y1: 32.768KHz, Crystal:Crystal_C26-LF_D2.1mm_L6.5mm_Horizontal_1EP_style1, F.Cu at (219.8, 66.8)
- added Y2: 8MHz, Crystal:Crystal_SMD_HC49-SD, F.Cu at (113.8, 70.1)
- added Y2: 8MHz, Crystal:Crystal_SMD_HC49-SD, F.Cu at (227.4, 70.1)
- added Y2: 8MHz, Crystal:Crystal_SMD_HC49-SD, F.Cu at (113.8, 135.1)
- J4: footprint Connector_PinHeader_2.54mm:PinHeader_2x01_P2.54mm_Vertical -> Connector_PinHeader_2.54mm:PinHeader_1x02_P2.54mm_Vertical_SMD_Pin1Right
- moved J4 67.9 mm to (215.1, 122.6), turned to 0 degrees
- moved C27 67.3 mm to (217.6, 126.8)
- moved D12 67.3 mm to (219.4, 126.8)
- moved D13 67.3 mm to (221.4, 126.8)
- moved C1 67.1 mm to (191.9, 116.6)
- moved C12 67.1 mm to (207.6, 119.8)
- moved C29 67.1 mm to (223.8, 132.6)
- moved C3 67.1 mm to (191.9, 112.1)
- moved C30 67.1 mm to (223.8, 129.4)
- moved C31 67.1 mm to (223.8, 136.7)
- moved R2 67.1 mm to (191.9, 118.2)
- moved R4 67.1 mm to (191.9, 115.1)
- moved R6 67.1 mm to (191.9, 113.6)
- moved R7 67.1 mm to (191.9, 110.5)
- moved U5 67.1 mm to (207.1, 132.4)
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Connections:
- J5 pad 1: PWM LED -> PWM
- U6 pad 32: PWM LED -> unconnected-(U6-Pad32)
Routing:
- net GND: track 280.2 -> 1124.4 mm, vias 10 -> 40
- net +3V3: track 269.1 -> 1059.3 mm, vias 5 -> 16
- net +5V: track 180.2 -> 716.4 mm, vias 5 -> 20
- net Net-(C26-Pad1): track 110.9 -> 458.3 mm, vias 2 -> 8
- net +24V: track 82.9 -> 331.6 mm, vias 1 -> 4
- net Tip_Temp: track 77.7 -> 326.0 mm, vias 2 -> 8
- net Handle_Temp: track 71.5 -> 301.3 mm, vias 2 -> 8
- net Vibra Sensor: track 65.2 -> 262.3 mm, vias 1 -> 4
- net PWM: track 31.7 -> 216.8 mm, vias 2 -> 16
- net Voltage: track 61.7 -> 246.7 mm, vias 2 -> 8
- net Current: track 53.0 -> 211.9 mm, vias 2 -> 8
- net Net-(C4-Pad1): track 37.8 -> 153.7 mm
- net ESP_Rx: track 32.9 -> 131.6 mm
- net ESP_Tx: track 32.1 -> 128.4 mm
- net HEAT_WIRE: track 32.1 -> 128.4 mm, vias 1 -> 4
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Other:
- board size 86.5 x 47.4 mm -> 200.1 x 112.3 mm
- board text added: "Designed by MVA"
